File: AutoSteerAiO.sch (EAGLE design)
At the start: 81 parts, among them IC2 MMA8452Q, J4 CONNECTOR 1x5 PINS, K4 CB1A-P-12V, U1 VX7805-1000

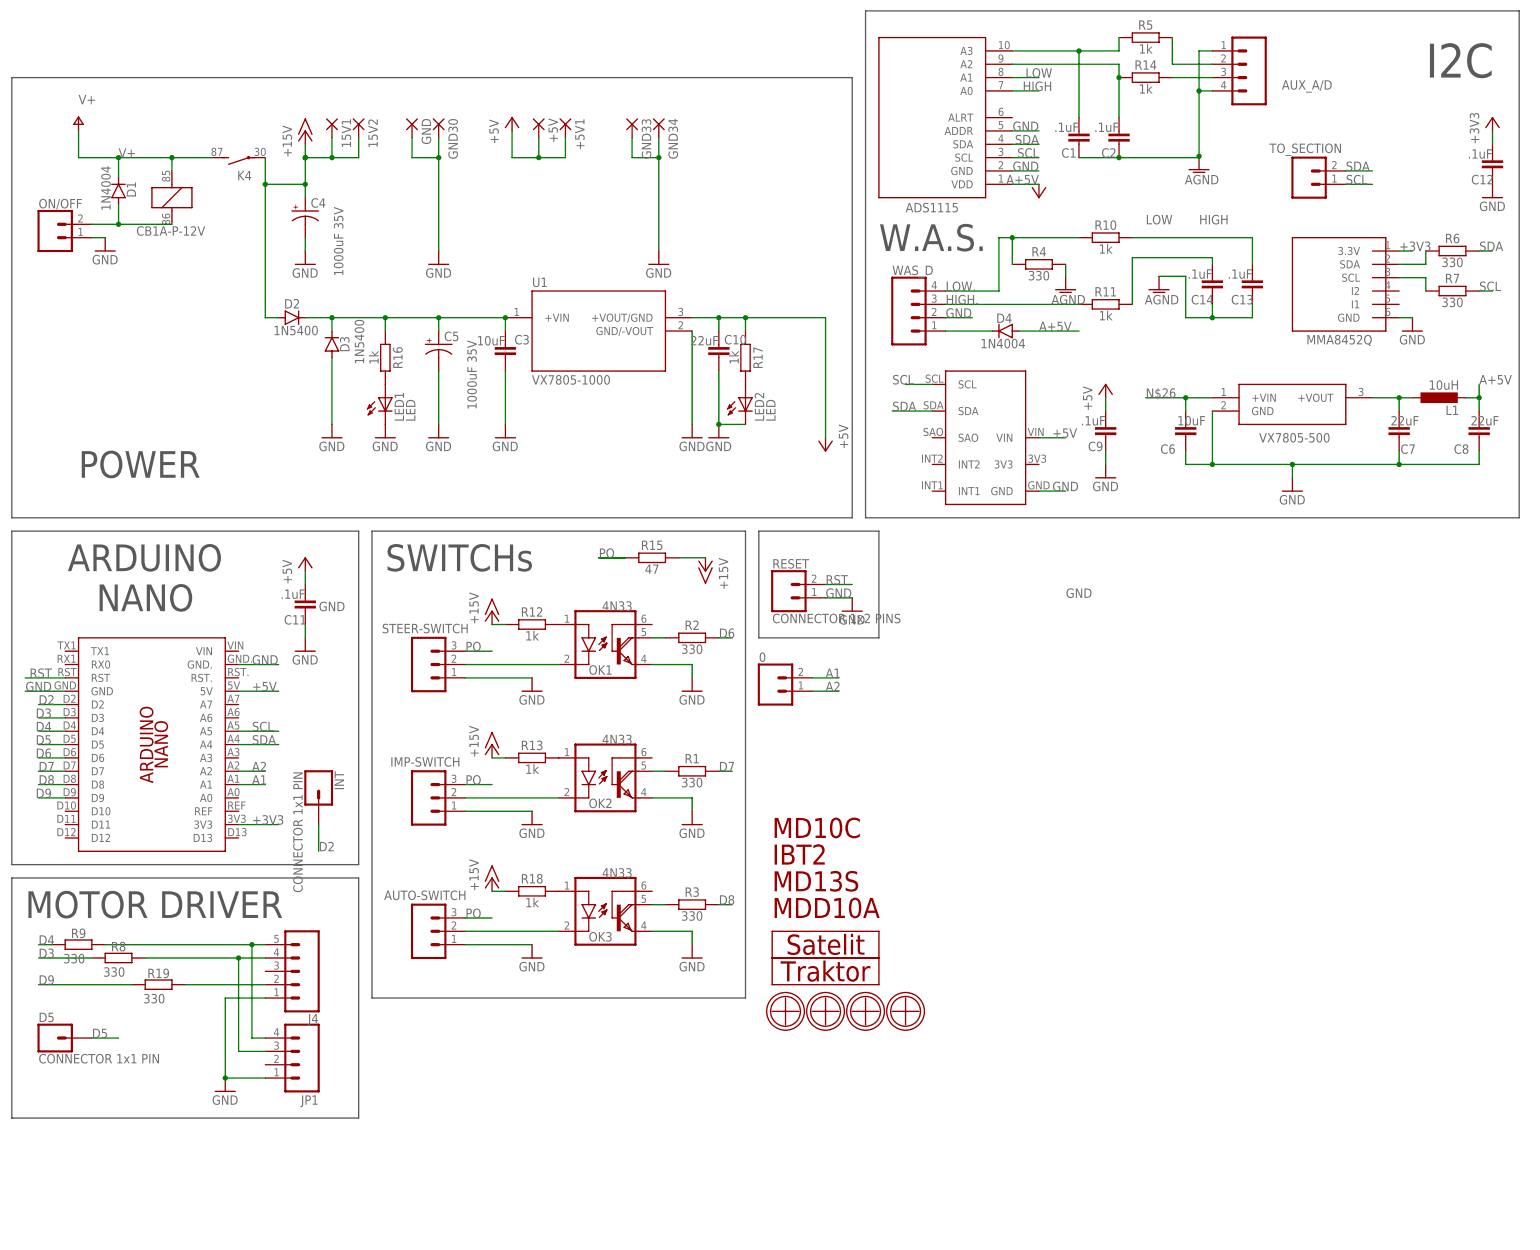
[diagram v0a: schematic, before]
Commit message: Add files via upload
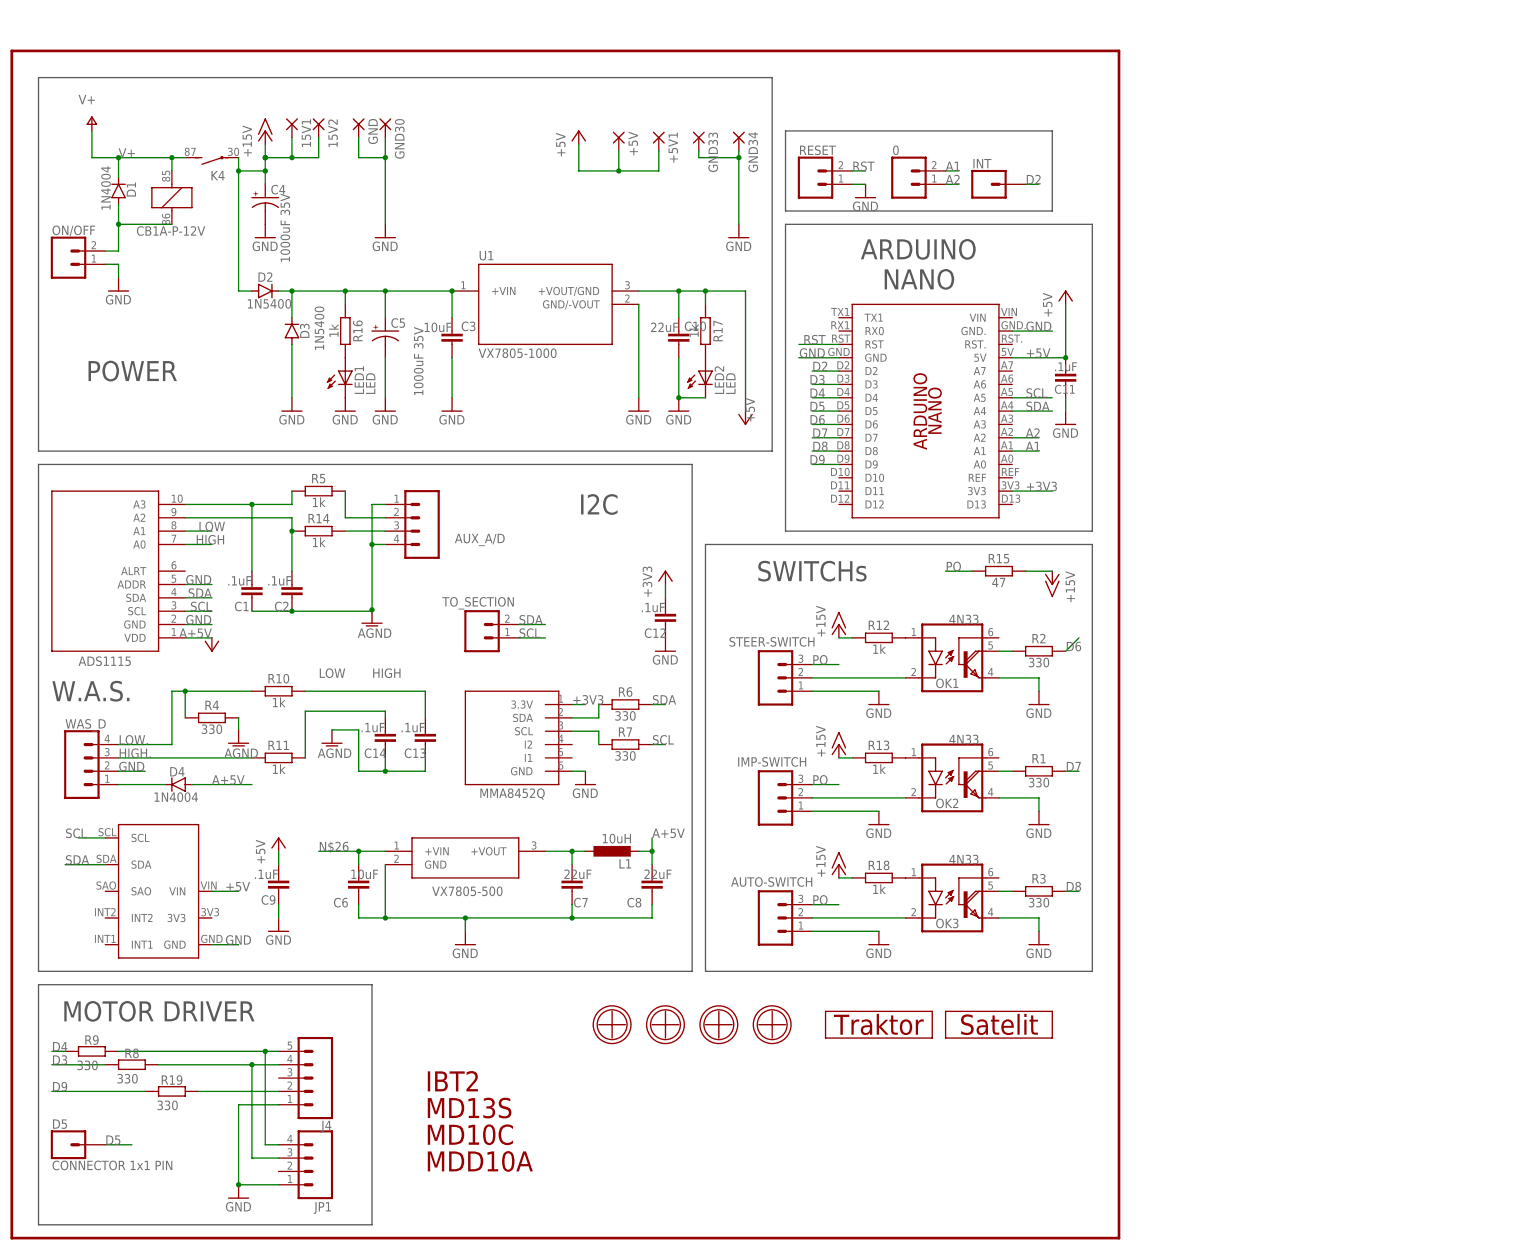
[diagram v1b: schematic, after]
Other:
- moved on the sheet: +5V, +5V1, 0, 15V1, 15V2, ADS1115, AUTO-SWITCH, AUX_A/D, C1, C10, C11, C12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
